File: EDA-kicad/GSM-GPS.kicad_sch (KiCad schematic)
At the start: 2 parts, among them J3 SIM-G85D1160022HHR, U9 GSM-GPS-EC25VFA-512-STD

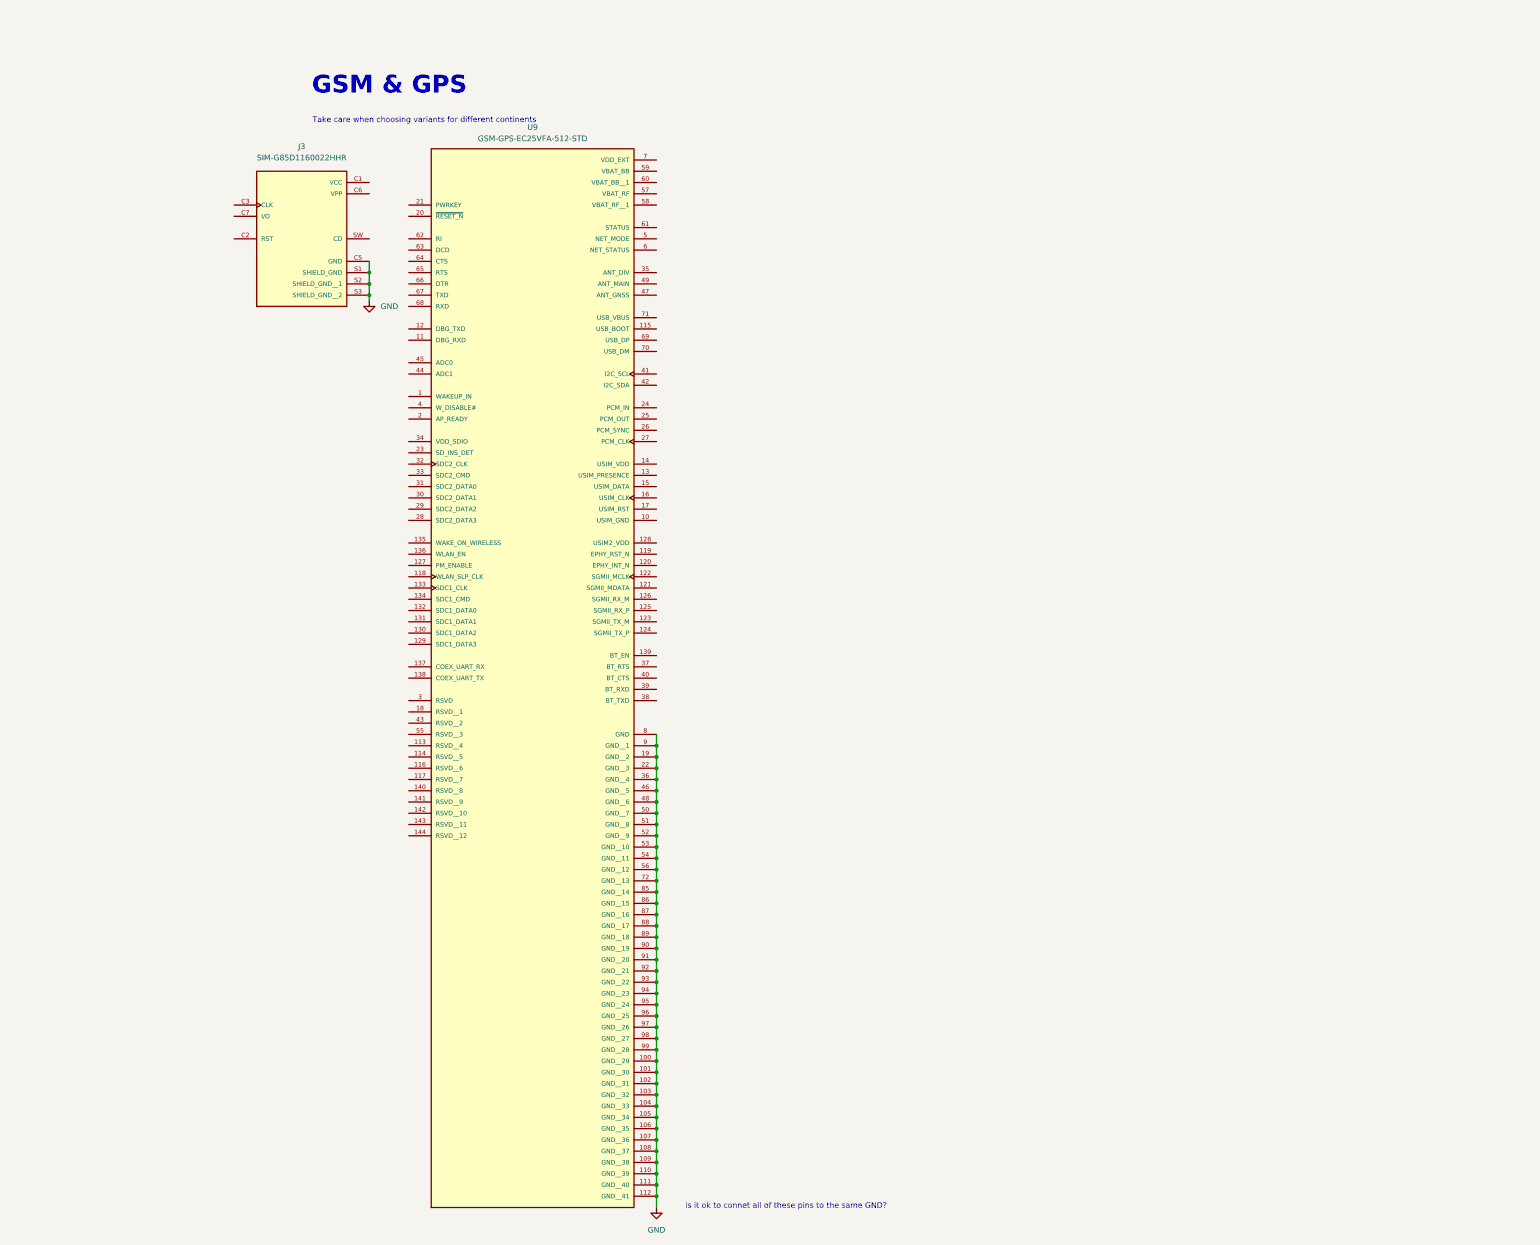
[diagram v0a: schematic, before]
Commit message: add EG25 new gpsgsm
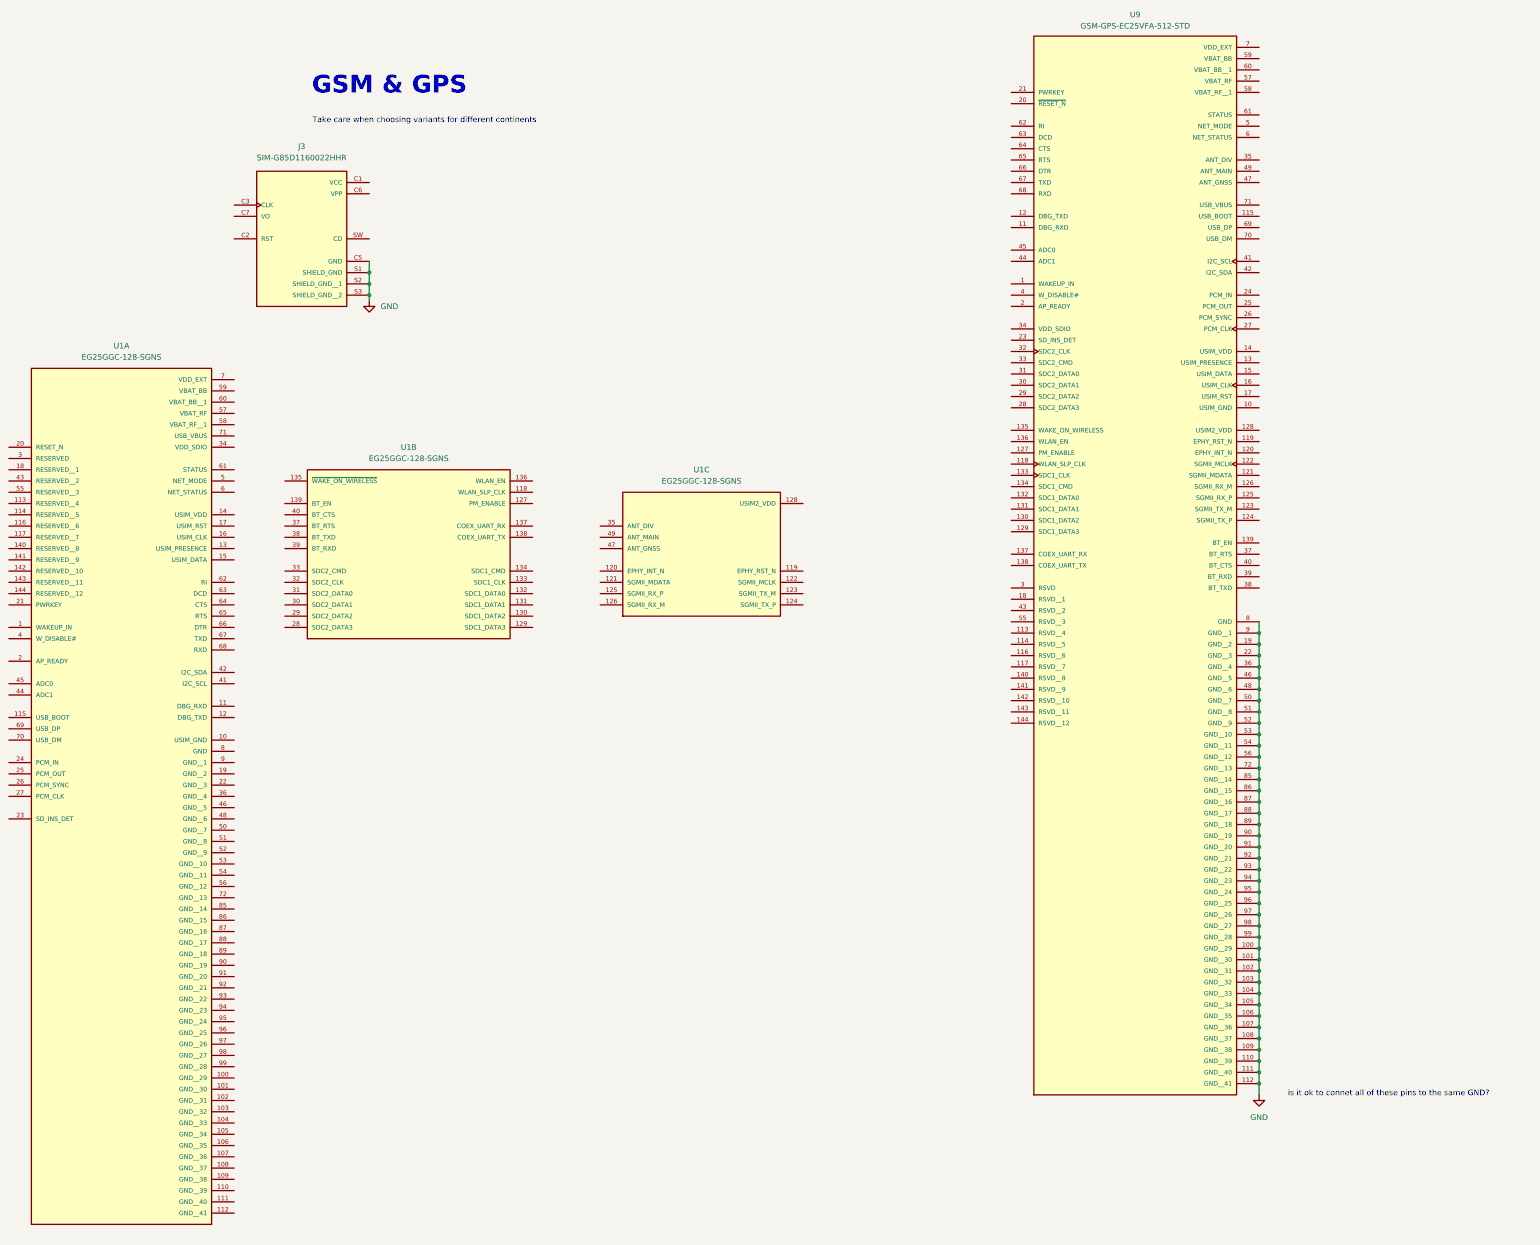
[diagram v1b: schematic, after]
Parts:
- added U1: EG25GGC-128-SGNS, SPIRIT-footprints:XCVR_EG25GGC-128-SGNS, symbol SPIRIT-components:EG25GGC-128-SGNS
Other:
- moved on the sheet: U9
